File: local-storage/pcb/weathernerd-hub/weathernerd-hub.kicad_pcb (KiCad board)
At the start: 2 copper layers, 80 x 60 mm, 15 parts, among them J1 WindNerd-Conn, Q1 2N7002, Q2 AO3401, U1 ESP32-C6-SuperMini, U2 MicroSD-SPI, U3 BME280, U4 DS3231, U5 OLED-Encoder-Btns

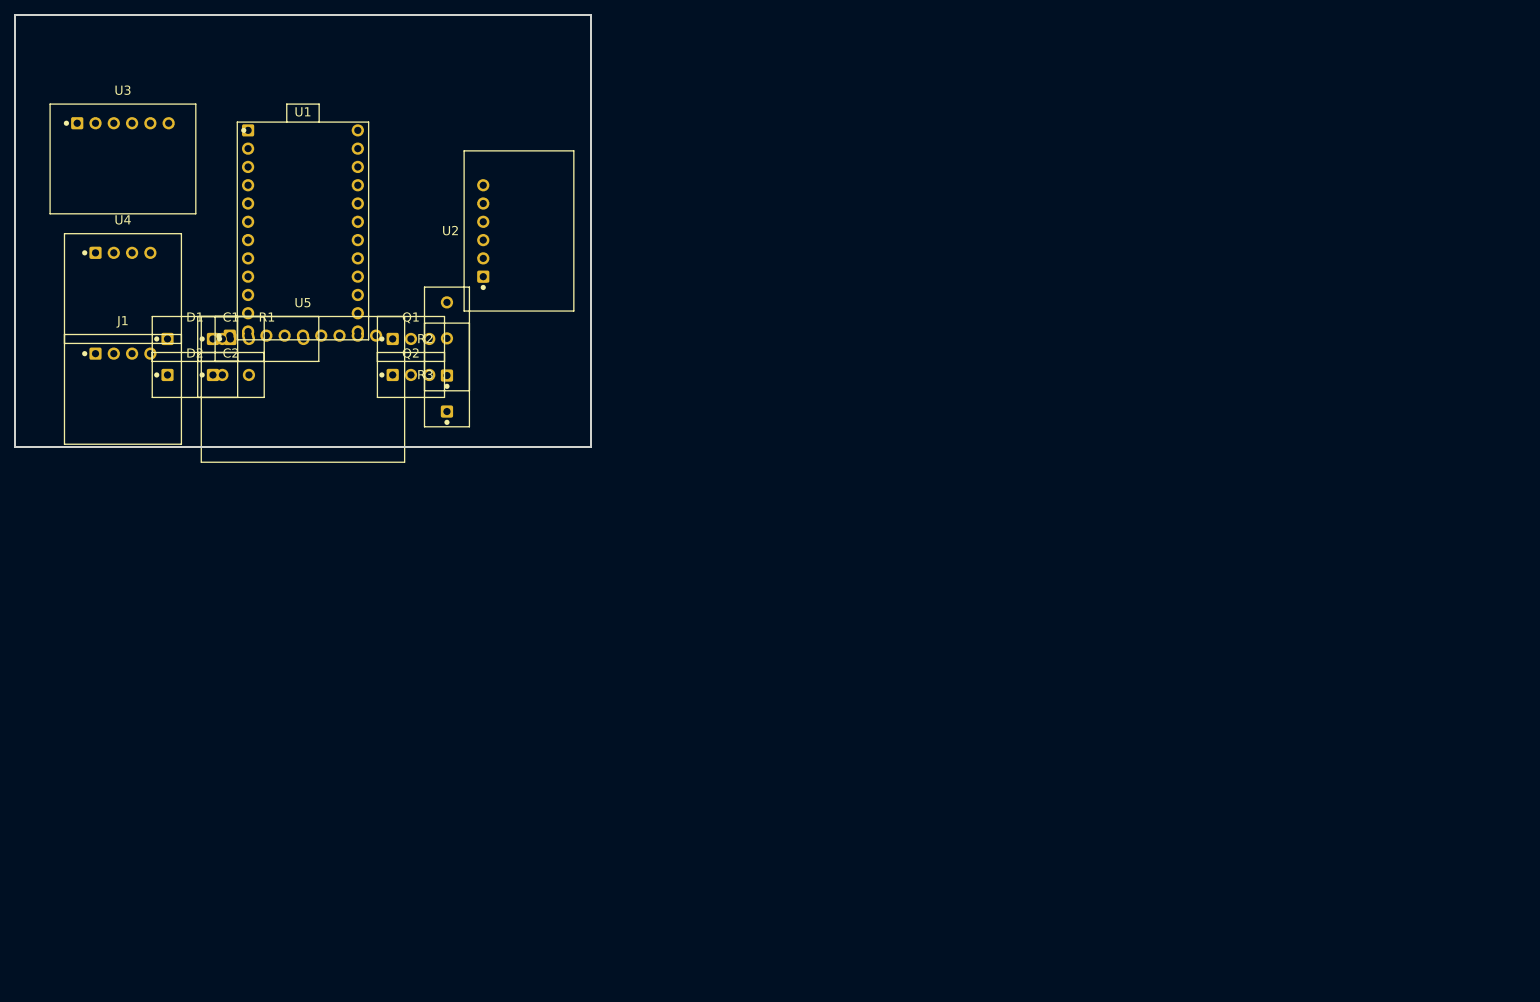
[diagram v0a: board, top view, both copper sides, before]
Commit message: the start of a human touch
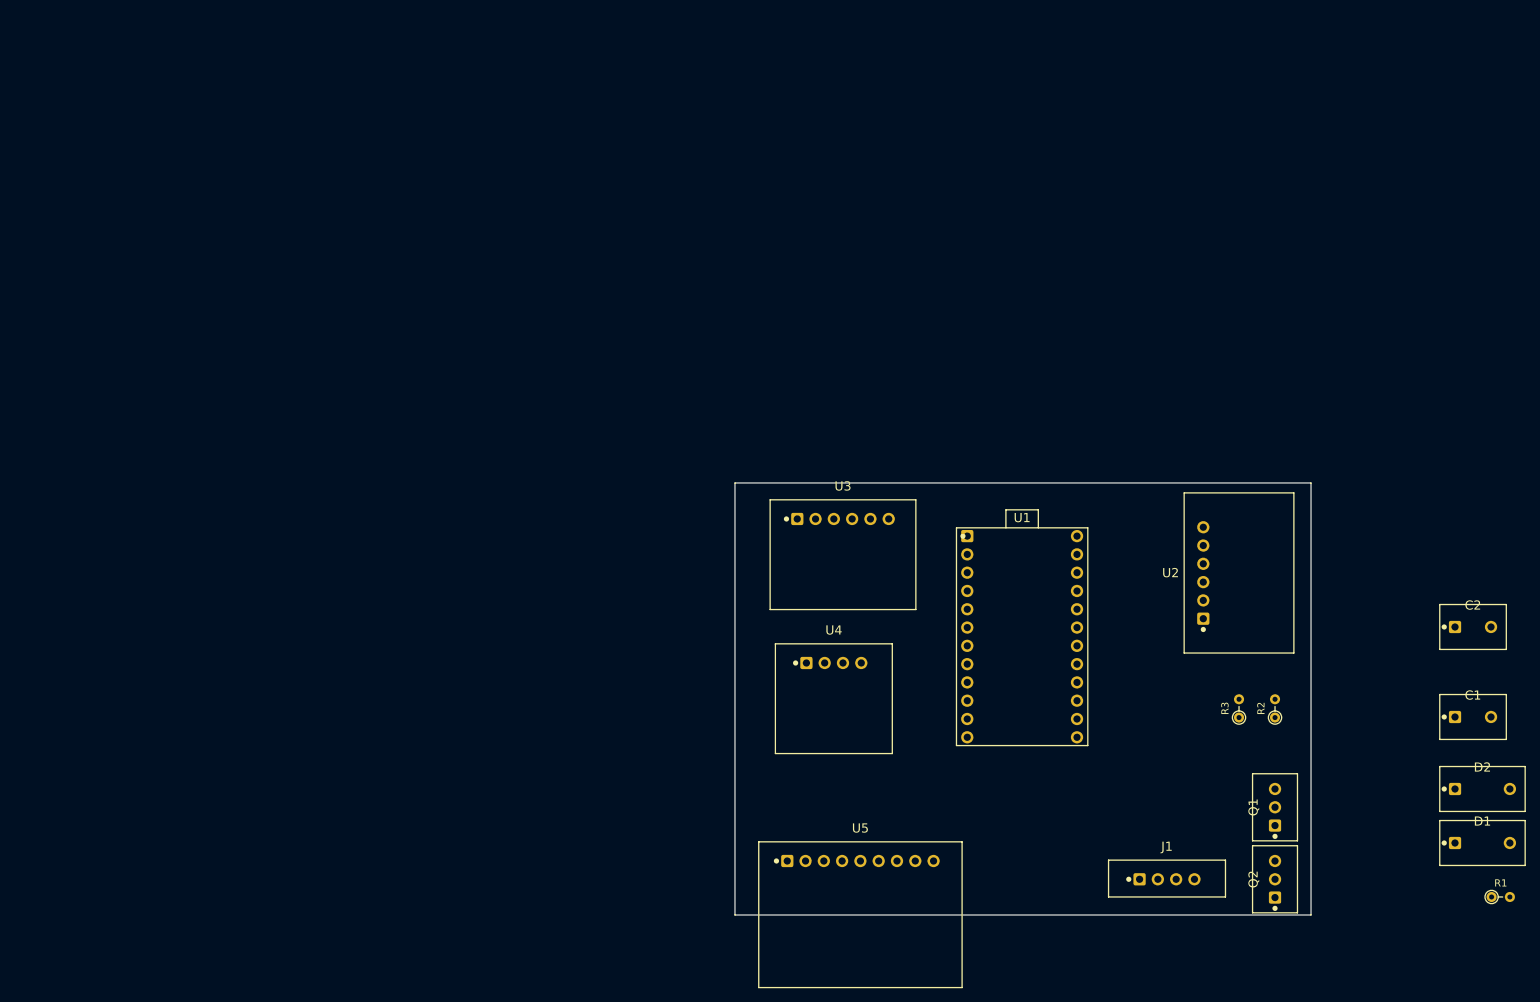
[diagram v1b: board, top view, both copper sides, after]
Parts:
- J1: footprint WindNerd-Conn -> weathernerd:WindNerd-Conn
- R1: footprint THT:R1 -> Resistor_THT:R_Axial_DIN0204_L3.6mm_D1.6mm_P2.54mm_Vertical
- R2: footprint THT:R2 -> Resistor_THT:R_Axial_DIN0204_L3.6mm_D1.6mm_P2.54mm_Vertical
- R3: footprint THT:R3 -> Resistor_THT:R_Axial_DIN0204_L3.6mm_D1.6mm_P2.54mm_Vertical
- moved D1 192.0 mm to (203.8, 115.0)
- moved D2 187.8 mm to (203.8, 107.5)
- moved R1 186.9 mm to (205.1, 122.5)
- moved C1 180.3 mm to (202.5, 97.5)
- moved C2 176.0 mm to (202.5, 85.0)
- moved J1 162.3 mm to (160.0, 125.0)
- moved Q2 138.9 mm to (175.0, 120.0), turned to 90 degrees
- moved Q1 136.5 mm to (175.0, 110.0), turned to 90 degrees
- moved R2 126.5 mm to (175.0, 97.6)
- moved R3 119.8 mm to (170.0, 97.6)
- moved U1 114.7 mm to (139.9, 86.3)
- moved U3 114.1 mm to (115.0, 75.0)
- moved U4 114.0 mm to (113.7, 95.0)
- moved U2 110.7 mm to (170.0, 77.5)
- moved U5 106.4 mm to (117.4, 125.0)
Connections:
- C1 pad 1: (no net) -> Net-(D1-K)
- C1 pad 2: (no net) -> unconnected-(C1-Pad2)
- C2 pad 1: (no net) -> PEAK
- C2 pad 2: (no net) -> GND
- J1 pad GND: (no net) -> GND
- J1 pad RX: (no net) -> WIND_TX
- J1 pad TRG: (no net) -> WIND_TRIG
- J1 pad VCC: (no net) -> +3V3
- Q1 pad D: (no net) -> PEAK
- Q1 pad G: (no net) -> RAIN_RST
- Q1 pad S: (no net) -> GND
- Q2 pad D: (no net) -> OLED_PWR
- Q2 pad G: (no net) -> OLED_GATE
- Q2 pad S: (no net) -> +3V3
- R1 pad 1: (no net) -> PEAK
- R1 pad 2: (no net) -> RAIN_ADC
- R2 pad 1: (no net) -> RAIN_RST
- R2 pad 2: (no net) -> GND
- R3 pad 1: (no net) -> OLED_GATE
- R3 pad 2: (no net) -> +3V3
- U1 pad 0: (no net) -> RAIN_ADC
- U1 pad 1: (no net) -> WIND_TRIG
- U1 pad 12: (no net) -> unconnected-(U1-IO12-Pad12)
- U1 pad 13: (no net) -> unconnected-(U1-IO13-Pad13)
- U1 pad 14: (no net) -> ENC_A
- U1 pad 15: (no net) -> unconnected-(U1-IO15-Pad15)
- U1 pad 16: (no net) -> unconnected-(U1-IO16-Pad16)
- U1 pad 17: (no net) -> unconnected-(U1-IO17-Pad17)
- U1 pad 18: (no net) -> SPI_MOSI
- U1 pad 19: (no net) -> SPI_MISO
- U1 pad 2: (no net) -> SPI_SCK
- U1 pad 20: (no net) -> ENC_B
- U1 pad 22: (no net) -> CON_BTN
- U1 pad 23: (no net) -> BAK_BTN
- U1 pad 3: (no net) -> SPI_CS
- U1 pad 3V3: (no net) -> +3V3
- U1 pad 4: (no net) -> WIND_TX
- U1 pad 5: (no net) -> OLED_GATE
- U1 pad 5V: (no net) -> unconnected-(U1-Pad5V)
- U1 pad 6: (no net) -> I2C_SDA
- U1 pad 7: (no net) -> I2C_SCL
- U1 pad 8: (no net) -> RAIN_RST
- U1 pad 9: (no net) -> unconnected-(U1-IO9-Pad9)
- U1 pad GND: (no net) -> GND
- U2 pad 3V3: (no net) -> +3V3
- U2 pad CLK: (no net) -> unconnected-(U2-PadCLK)
- U2 pad CS: (no net) -> SPI_CS
- U2 pad GND: (no net) -> GND
- U2 pad MISO: (no net) -> SPI_MISO
- U2 pad MOSI: (no net) -> SPI_MOSI
- U3 pad CSB: (no net) -> unconnected-(U3-PadCSB)
- U3 pad GND: (no net) -> GND
- U3 pad SCL: (no net) -> I2C_SCL
- U3 pad SDA: (no net) -> I2C_SDA
- U3 pad SDO: (no net) -> unconnected-(U3-PadSDO)
- U3 pad VCC: (no net) -> +3V3
- U4 pad GND: (no net) -> GND
- U4 pad SCL: (no net) -> I2C_SCL
- U4 pad SDA: (no net) -> I2C_SDA
- U4 pad VCC: (no net) -> +3V3
- U5 pad BAK: (no net) -> BAK_BTN
- U5 pad CON: (no net) -> CON_BTN
- U5 pad GND: (no net) -> GND
- U5 pad PSH: (no net) -> ENC_PSH
- U5 pad SCL: (no net) -> I2C_SCL
- U5 pad SDA: (no net) -> I2C_SDA
- U5 pad TRA: (no net) -> ENC_A
- U5 pad TRB: (no net) -> ENC_B
- U5 pad VCC: (no net) -> OLED_PWR
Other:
- net class Default removed
